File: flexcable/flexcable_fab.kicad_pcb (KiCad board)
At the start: 2 copper layers, 80.2 x 35.1 mm, 12 parts, among them J1 Molex 200528_0400, J2 TWL_DCap_V12, J3 TWL_DCap_GND, J4 Molex 200528_0400, J5 UTL_DCap_V12, J6 UTL_DCap_GND, J7 UTL_DCap_V12, J8 UTL_DCap_GND, Q1 IRFHS8342PbF, Q2 IRFHS8342PbF

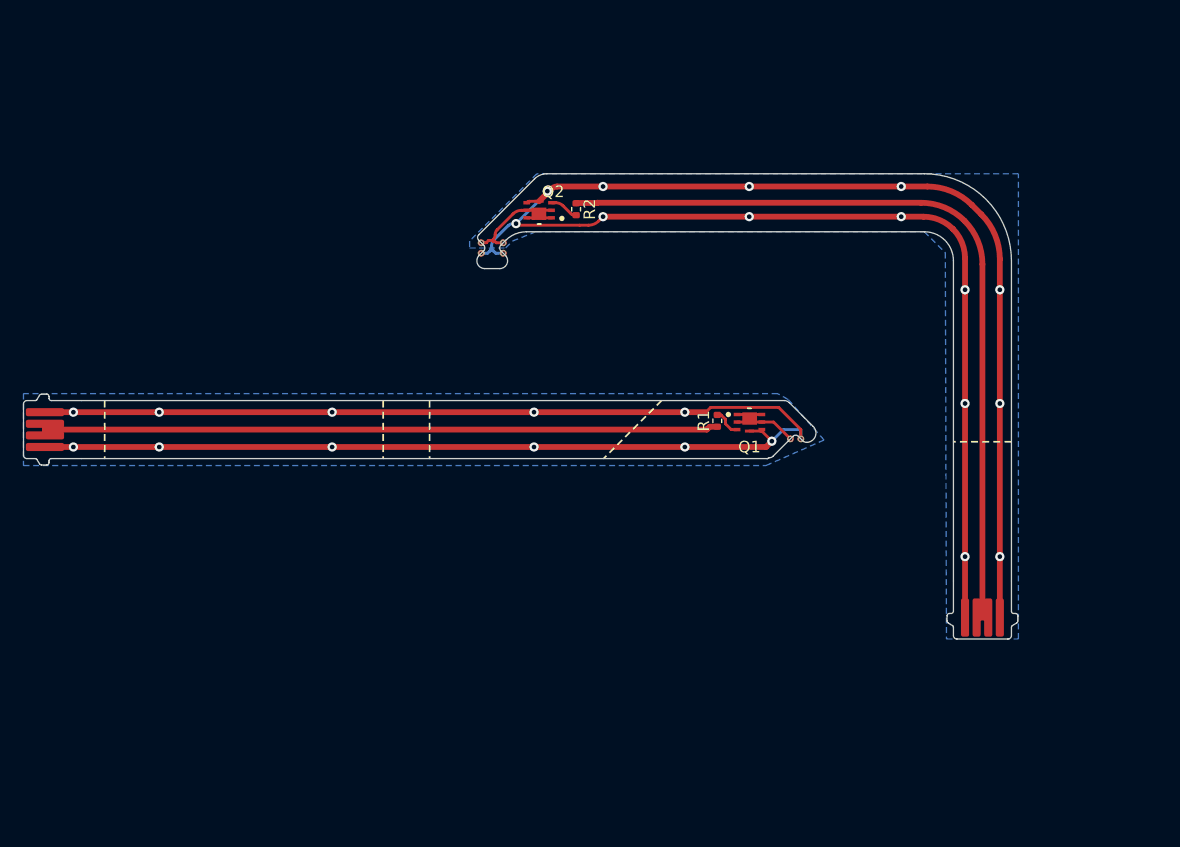
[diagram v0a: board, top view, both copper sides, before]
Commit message: version ready-ish for fabrication
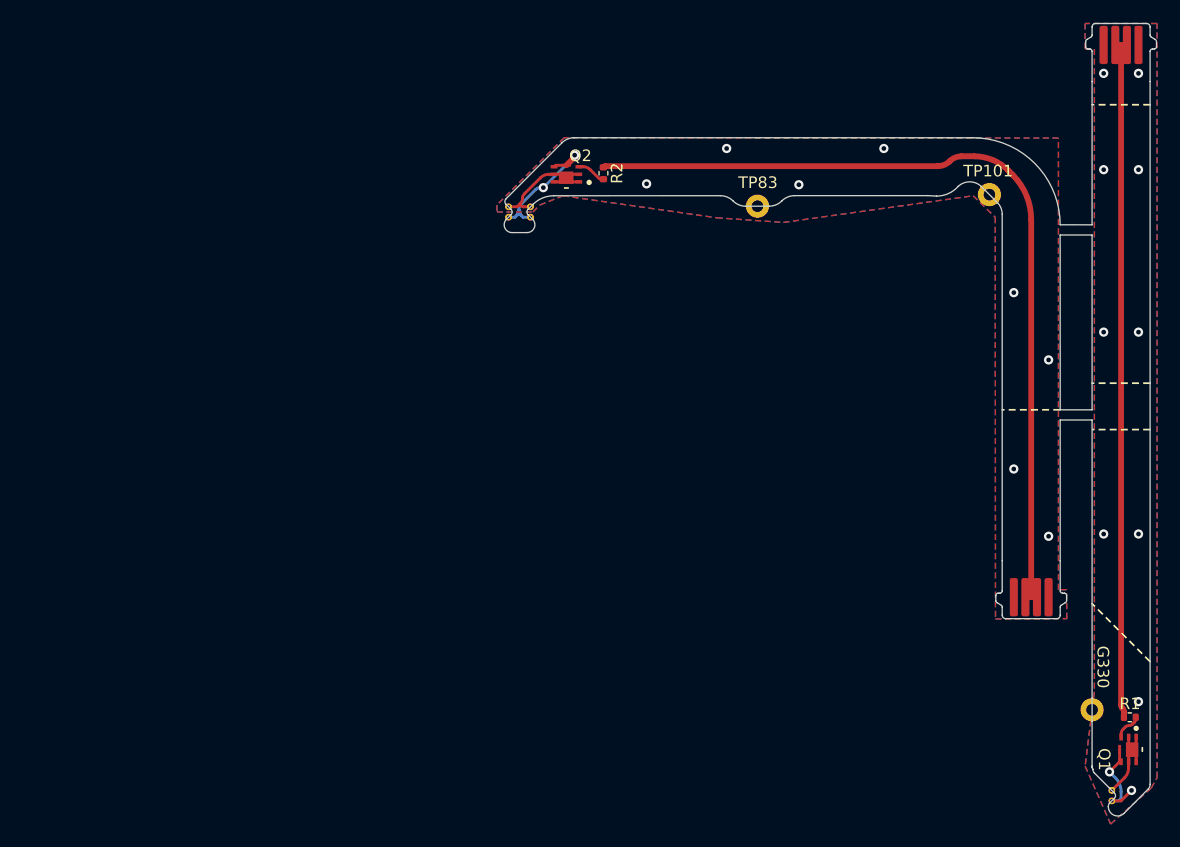
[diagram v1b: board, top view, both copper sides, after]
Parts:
- added H1: TWL_GPIO330, footprints:TestPointAnchor_D1.00, F.Cu at (232.0, 115.2)
- added H2: UTL_TP83_PENIRQ, footprints:TestPointAnchor_D1.00, F.Cu at (203.2, 71.7)
- added H3: UTL_TP101_HP#SP, footprints:TestPointAnchor_D1.00, F.Cu at (223.2, 70.7)
- moved J1 94.5 mm to (234.5, 61.0), turned to 0 degrees
- moved R1 43.8 mm to (235.3, 115.8), turned to 0 degrees
- moved Q1 43.2 mm to (235.1, 118.6), turned to -90 degrees
- moved J3 41.1 mm to (233.7, 123.0), turned to -135 degrees
- moved J2 41.1 mm to (233.7, 122.1), turned to -45 degrees
- moved J4 4.55 mm to (226.8, 102.3)
- moved J5 3.89 mm to (181.7, 71.8)
- moved J6 3.89 mm to (181.7, 72.7)
- moved J7 3.89 mm to (183.6, 71.8)
- moved Q2 3.89 mm to (186.7, 69.0)
- moved R2 3.89 mm to (189.9, 68.9)
- moved J8 3.89 mm to (183.6, 72.7)
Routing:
- net GND: track 293.6 -> 20.4 mm, vias 25 -> 21
- net /G_UTL: track 70.0 -> 74.3 mm
- net +1V2: track 15.2 -> 17.4 mm
- added copper zone on F.Cu, net GND
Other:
- board size 80.2 x 35.1 mm -> 55.7 x 63.3 mm
- board text added: "G330"
- board text added: "TP101"
- board text added: "TP83"
- board text added: "User.4 = stiffner outline PI stiffner, T=0.3mm *total* => 0.11mm FPC, 0.25mm stiffener stiffner on bottom side"
- board text added: "custom layers: * User.1 = stiffner meta/info * User.4 = stiffner outline/shape"
- board text removed: "2nd fold (90°)"
- board text removed: "3rd fold (90°)"
- board text removed: "4th fold (180°, diag)"
- board text removed: "User.4 = stiffner outline PI stiffner, T=0.3mm *total*"
- board text removed: "custom layers: * User.1 = stiffner meta * User.4 = stiffner outline"
- board text removed: "first fold (180°)"
